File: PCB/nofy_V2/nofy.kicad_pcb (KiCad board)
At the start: 2 copper layers, 205.6 x 171.6 mm, 147 parts, among them J10 Conn_01x01-Connector_Generic, J11 Conn_01x01-Connector_Generic, J13 Conn_01x01-Connector_Generic, J14 Conn_01x01-Connector_Generic, J15 Conn_01x01-Connector_Generic, J16 Conn_01x01-Connector_Generic, J17 Conn_01x01-Connector_Generic, J18 Conn_01x01-Connector_Generic, J19 Conn_01x01-Connector_Generic, J21 Conn_01x01-Connector_Generic, J22 PIn1x4, J23 PIn1x4, J24 PIn1x4, J25 PIn1x4, J26 PIn1x4, J27 PIn1x4, J28 PIn1x4, J29 PIn1x4, J30 PIn1x4, J31 PIn1x4, J32 PIn1x4, J33 PIn1x4, J34 PIn1x4, J35 PIn1x4, J36 PIn1x4, J37 PIn1x4, J38 PIn1x4, J39 PIn1x4, J40 PIn1x4, J41 PIn1x4, SW1 RotaryEncoder, SW10 SW_PUSH, SW11 SW_PUSH, SW12 SW_PUSH, SW13 SW_PUSH, SW14 SW_PUSH, SW15 SW_PUSH, SW16 SW_PUSH, SW17 SW_PUSH, SW18 SW_PUSH, SW19 SW_PUSH, SW2 RotaryEncoder, SW20 SW_PUSH, SW21 SW_PUSH, SW22 SW_PUSH, SW23 SW_PUSH, SW24 SW_PUSH, SW25 SW_PUSH, SW26 SW_PUSH, SW27 SW_PUSH, SW28 SW_PUSH, SW29 SW_PUSH, SW3 SW_SPDT, SW30 SW_PUSH, SW31 SW_PUSH, SW32 SW_PUSH, SW33 SW_PUSH, SW34 SW_PUSH, SW35 SW_PUSH, SW36 SW_PUSH, SW37 SW_PUSH, SW38 SW_PUSH, SW39 SW_PUSH, SW4 SW_SPDT, SW40 SW_PUSH, SW41 SW_PUSH, SW42 SW_PUSH, SW43 SW_PUSH, SW44 SW_PUSH, SW45 SW_PUSH, SW46 SW_PUSH, SW47 SW_PUSH, SW48 SW_PUSH, SW49 SW_PUSH, SW5 SW_PUSH, SW50 SW_PUSH, SW51 SW_PUSH, SW52 SW_PUSH, SW53 SW_PUSH, SW54 SW_PUSH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

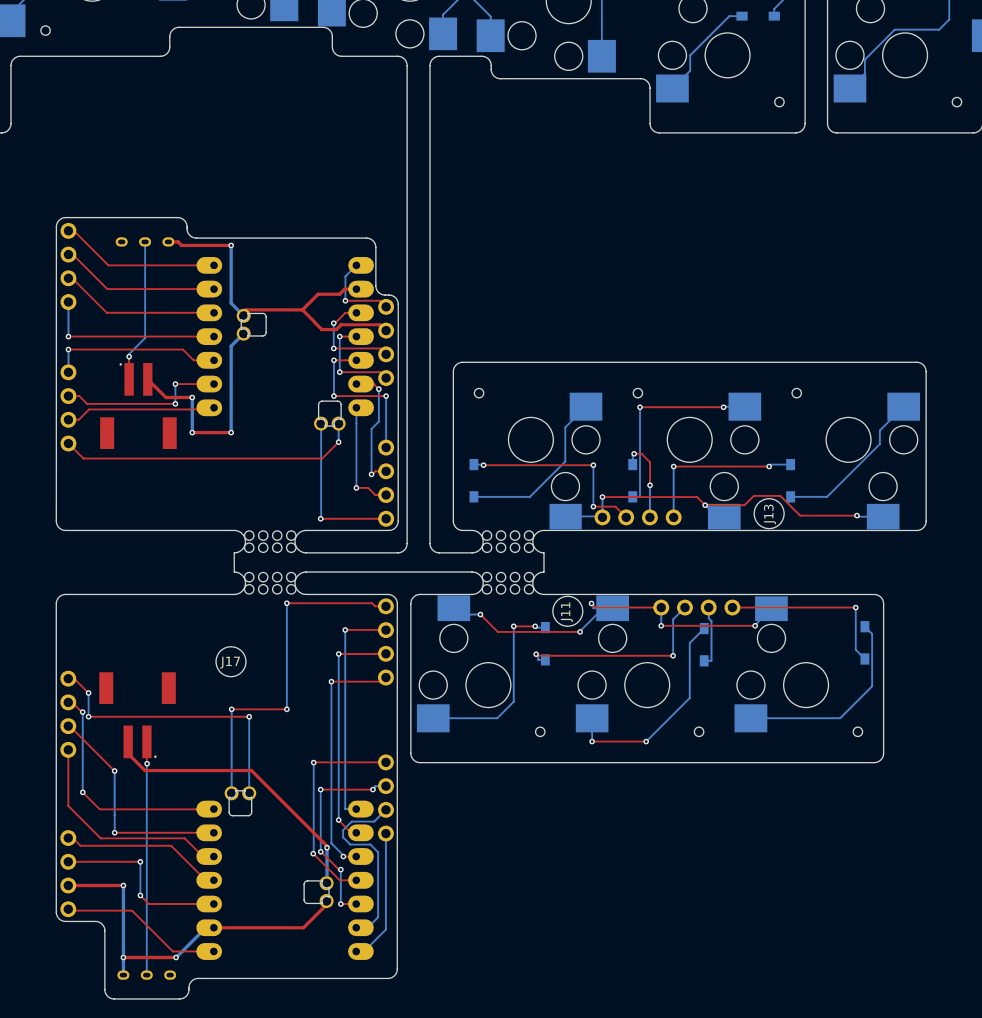
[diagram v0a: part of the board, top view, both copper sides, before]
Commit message: Update : PCB
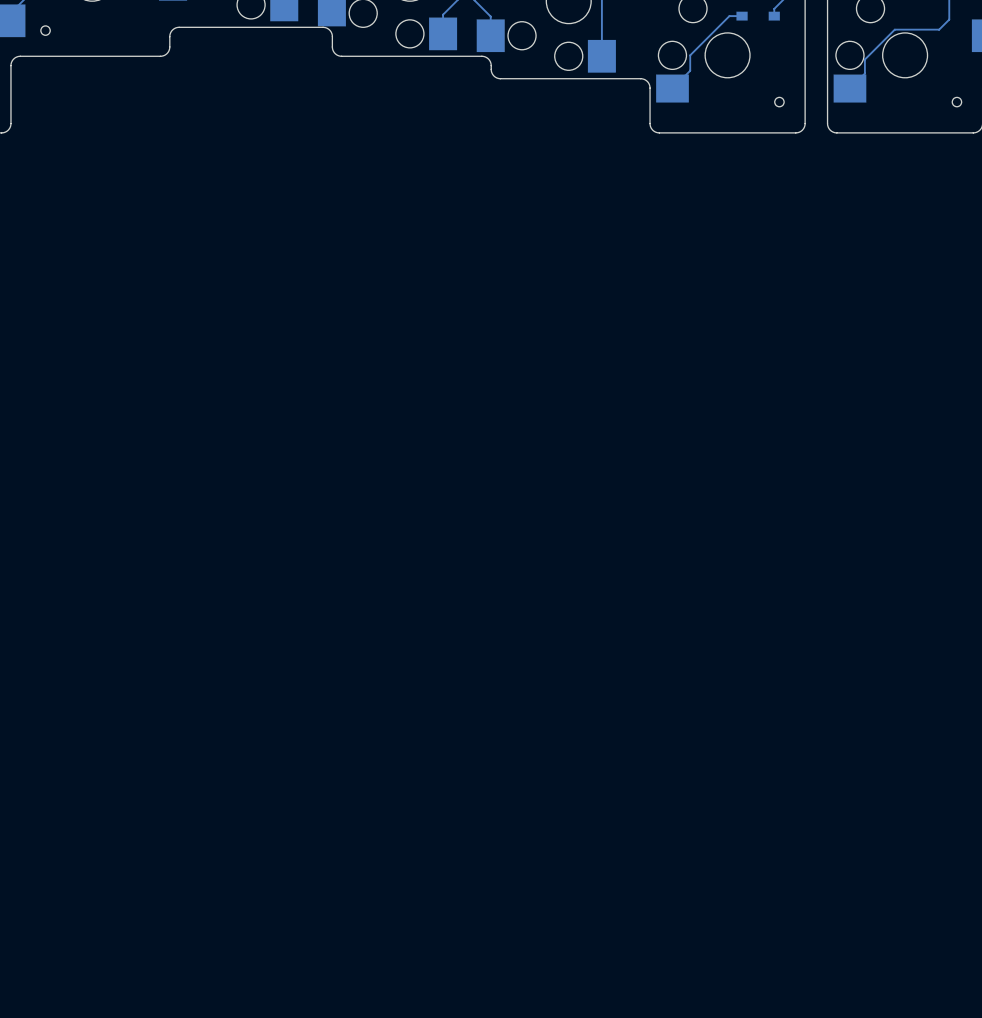
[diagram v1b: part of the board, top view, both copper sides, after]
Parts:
- removed B1: BATT_L, _kicad_footprints:JST_S2B-PH-SM4-TB
- removed BT1: BATT, _kicad_footprints:JST_S2B-PH-SM4-TB
- removed D22, D23, D24, D25, D26, D27: D, _kicad_footprints:Diode_SMD
- removed J11, J13, J17: Conn_01x01-Connector_Generic, MountingHole:MountingHole_3.2mm_M3
- removed J23, J24, J26, J28, J31, J33, J34, J35, J40, J41: PIn1x4, nofy:Pin1x4
- removed REF**2, REF**3, REF**4, REF**5: StampHole, nofy:StampHole
- removed SW26, SW27, SW28, SW29, SW30, SW31: SW_PUSH, nofy:Choc_v2_Hotswap_1u_17mm
- removed SW3, SW4: SW_SPDT, _kicad_footprints:TGSW_MSK-12D19
- removed U1, U2: ~, _kicad_footprints:XIAO_nRF52840_wBAT_wNFC_1
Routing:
- net Net-(J23-Pin_1): track 43.0 -> 0.00 mm, vias 5 -> 0
- net Net-(J24-Pin_1): track 40.7 -> 0.00 mm, vias 3 -> 0
- net GND_R_b: track 40.0 -> 0.00 mm, vias 3 -> 0
- net GND_L_b: track 38.8 -> 0.00 mm, vias 1 -> 0
- net Net-(J41-Pin_4): track 37.0 -> 0.00 mm, vias 3 -> 0
- net Net-(J33-Pin_4): track 32.3 -> 0.00 mm, vias 1 -> 0
- net Net-(J35-Pin_4): track 30.7 -> 0.00 mm, vias 3 -> 0
- net Bat: track 30.6 -> 0.00 mm, vias 1 -> 0
- net Net-(J41-Pin_1): track 26.6 -> 0.00 mm, vias 2 -> 0
- net Net-(J35-Pin_3): track 25.4 -> 0.00 mm, vias 2 -> 0
- net Net-(J41-Pin_2): track 25.3 -> 0.00 mm, vias 2 -> 0
- net Net-(BT1--): track 25.0 -> 0.00 mm, vias 1 -> 0
- net Net-(J41-Pin_3): track 24.7 -> 0.00 mm, vias 1 -> 0
- net Bat_L: track 24.6 -> 0.00 mm, vias 3 -> 0
- net Net-(J35-Pin_2): track 24.2 -> 0.00 mm, vias 2 -> 0
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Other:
- board size 205.6 x 171.6 mm -> 205.6 x 78.9 mm
- board text removed: "nofy Engine"
